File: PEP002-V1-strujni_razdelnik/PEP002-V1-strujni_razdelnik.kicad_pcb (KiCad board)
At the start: 2 copper layers, 45 x 45 mm, 22 parts, among them J1 Screw_Terminal_01x02

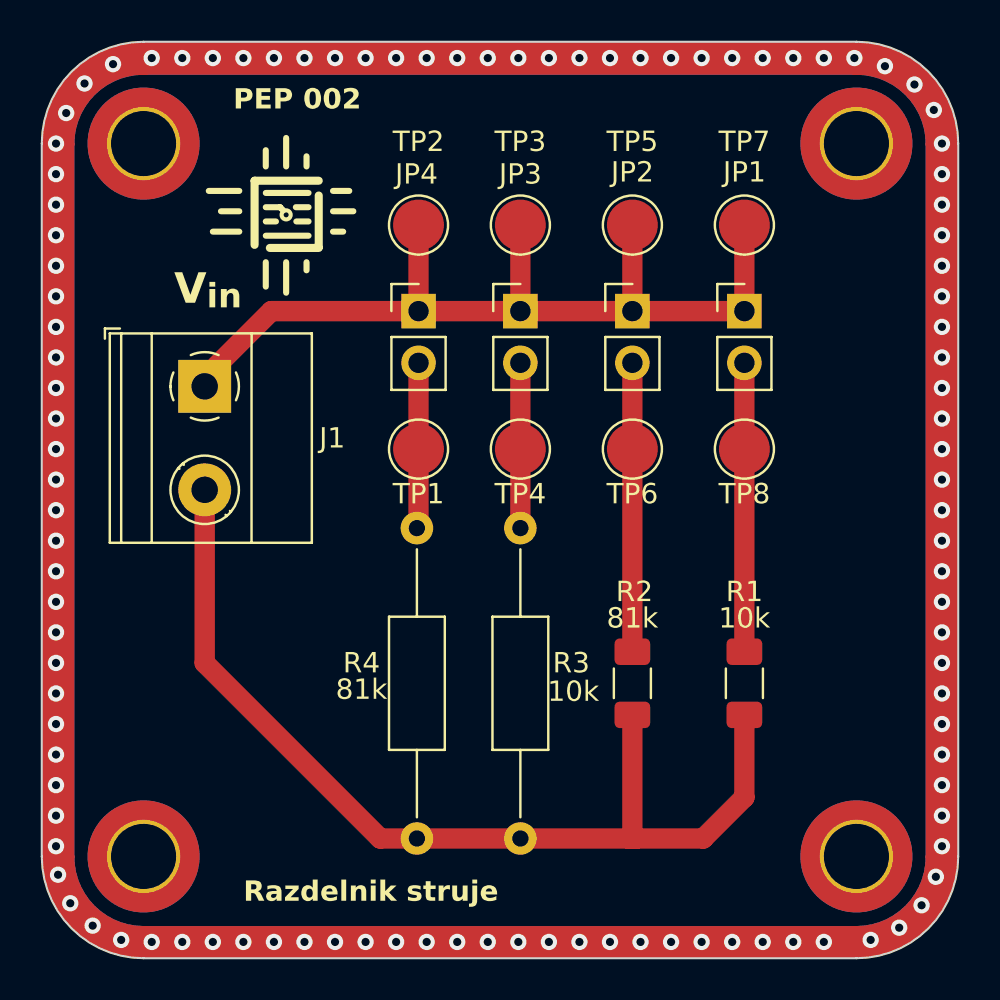
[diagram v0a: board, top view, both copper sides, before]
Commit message: Update 1,2,3,4,5,7, lib.
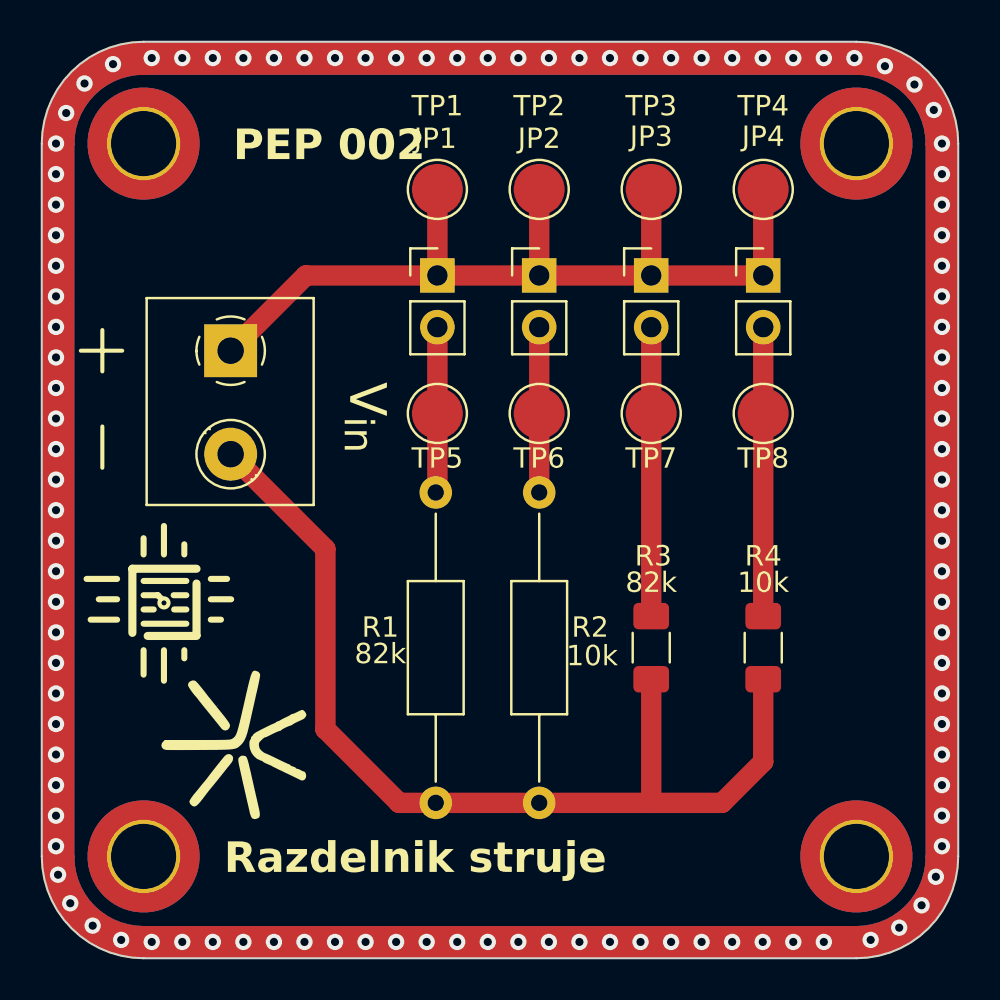
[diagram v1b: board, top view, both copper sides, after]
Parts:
- added G***: LOGO, PEP_library:petnica_logo, F.Cu at (113.5, 95.5)
- J1: footprint TerminalBlock_Phoenix:TerminalBlock_Phoenix_MKDS-1,5-2-5.08_1x02_P5.08mm_Horizontal -> PEP_library:TerminalBlock_Phoenix_MKDS-1,5-2-5.08_1x02_P5.08mm_Horizontal
- R1: renamed from R4; value 81k -> 82k
- R3: renamed from R2; value 81k -> 82k
- moved REF** 20.0 mm to (110.0, 88.6)
- moved J1 2.17 mm to (113.3, 76.2)
- moved JP2 1.98 mm to (128.4, 72.5)
- moved JP3 1.98 mm to (133.9, 72.5)
- moved JP4 1.98 mm to (139.4, 72.5)
- moved R2 1.98 mm to (128.4, 83.1)
- moved R3 1.98 mm to (133.9, 90.8)
- moved R4 1.98 mm to (139.4, 90.8)
- moved TP2 1.98 mm to (128.4, 68.2)
- moved TP3 1.98 mm to (133.9, 68.2)
- moved TP4 1.98 mm to (139.4, 68.2)
- moved TP6 1.98 mm to (128.4, 79.2)
- moved TP7 1.98 mm to (133.9, 79.2)
- moved TP8 1.98 mm to (139.4, 79.2)
- moved JP1 1.98 mm to (123.4, 72.5)
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- renumbered JP4 to JP1, JP3 to JP2, JP2 to JP3, JP1 to JP4, R3 to R2, R1 to R4, TP2 to TP1, TP3 to TP2, TP5 to TP3, TP7 to TP4, TP1 to TP5, TP4 to TP6, TP6 to TP7
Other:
- board text added: "JP1"
- board text added: "JP2"
- board text added: "JP3"
- board text added: "JP4"
- board text added: "R1"
- board text added: "R2"
- board text added: "R3"
- board text added: "R4"
- board text removed: "V_{in}"
